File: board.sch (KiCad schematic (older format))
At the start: 32 parts, among them J1 TEMPS, J2 OLED, J3 RELAY, J4 RELAY_EN, J5 USB_B_Micro, Q1 MMBT3904, Q2 MMBT3904, SW1 SW_RESET, U1 ESP32-WROOM-32, U2 AMS1117-3.3, U3 CP2104

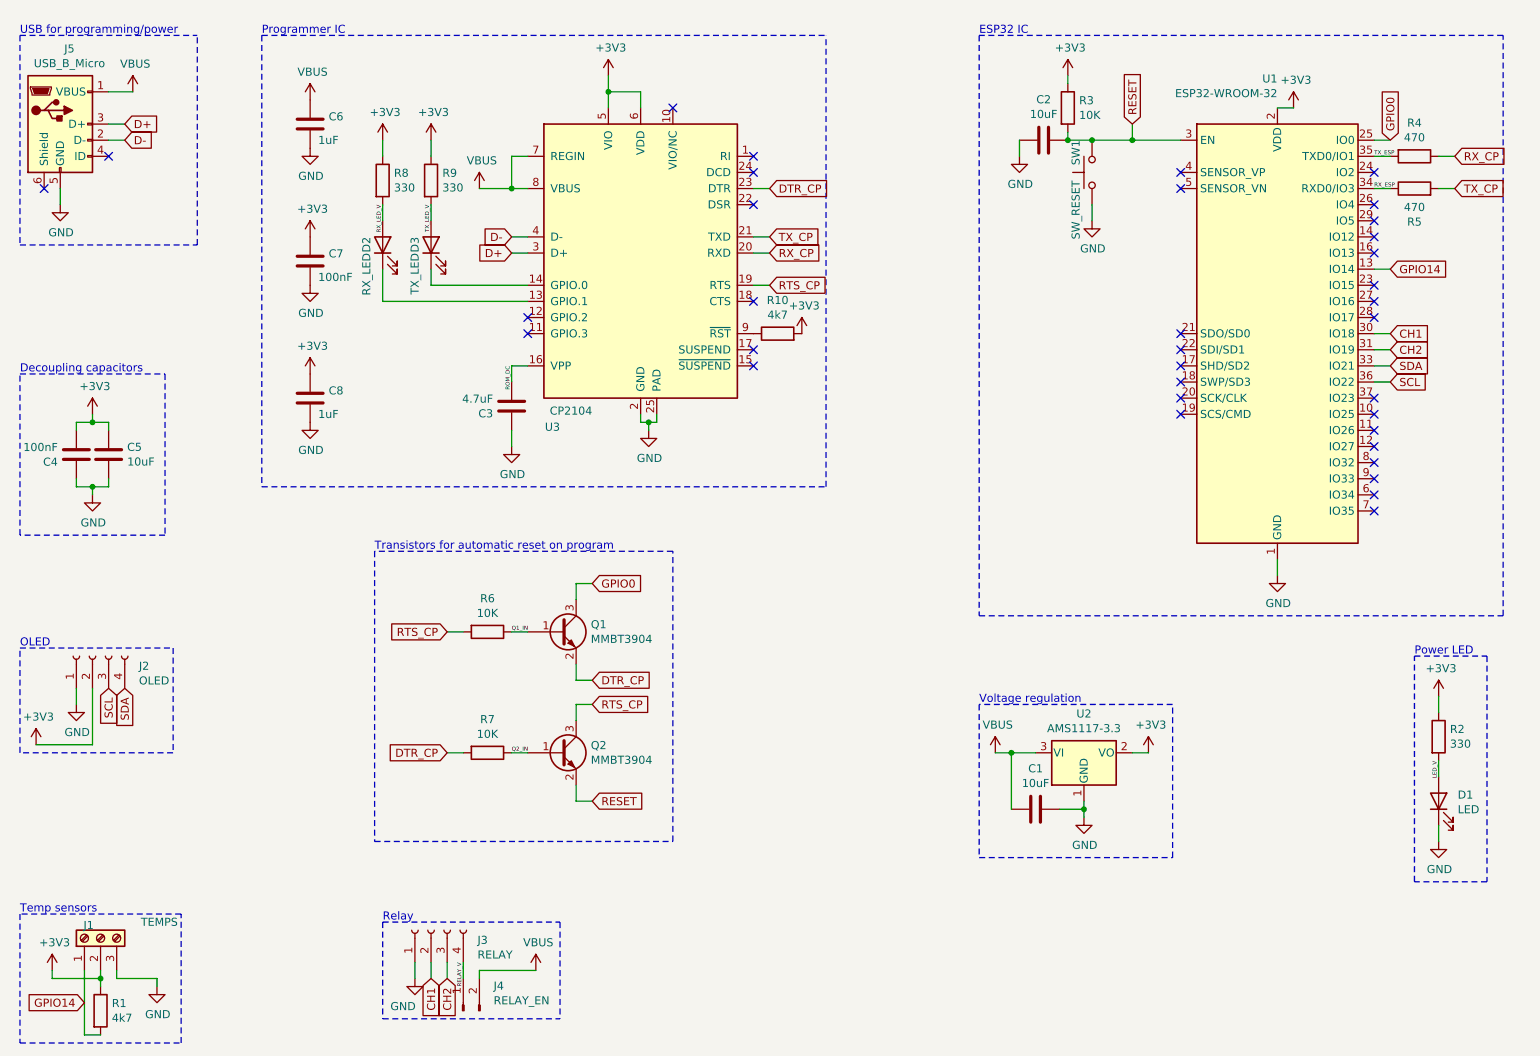
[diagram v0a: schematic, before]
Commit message: with programmer
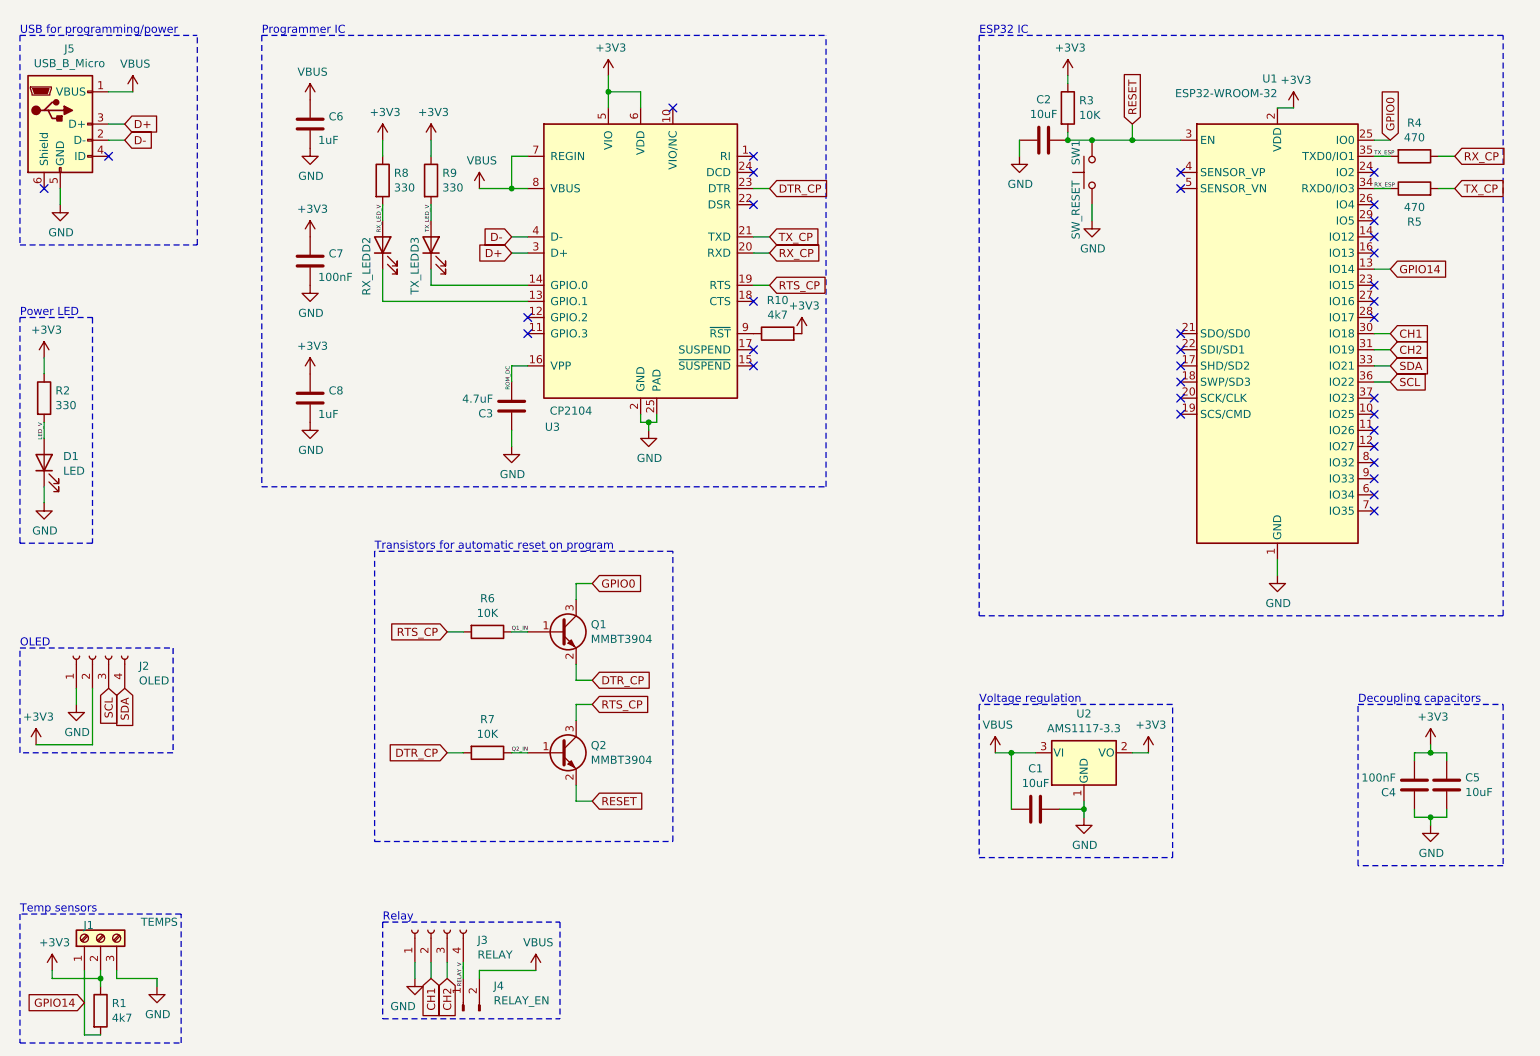
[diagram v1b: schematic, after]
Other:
- moved on the sheet: C4, C5, D1, R2
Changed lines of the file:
@@
 L Device:LED D1
 U 1 1 60E6779F
-P 9750 5700
-F 0 "D1" V 9789 5582 50  0000 R CNN
-F 1 "LED" V 9698 5582 50  0000 R CNN
-F 2 "LED_SMD:LED_0805_2012Metric" H 9750 5700 50  0001 C CNN
-F 3 "~" H 9750 5700 50  0001 C CNN
-	1    9750 5700
+P 1100 3600
+F 0 "D1" V 1139 3482 50  0000 R CNN
+F 1 "LED" V 1048 3482 50  0000 R CNN
+F 2 "LED_SMD:LED_0805_2012Metric" H 1100 3600 50  0001 C CNN
+F 3 "~" H 1100 3600 50  0001 C CNN
+	1    1100 3600
 	0    -1   -1   0
 $EndComp
@@
 L power:+3V3 #PWR01
 U 1 1 60E6985D
-P 9750 5050
-F 0 "#PWR01" H 9750 4900 50  0001 C CNN
-F 1 "+3V3" H 9765 5223 50  0000 C CNN
-F 2 "" H 9750 5050 50  0001 C CNN
-F 3 "" H 9750 5050 50  0001 C CNN
-	1    9750 5050
+P 1100 2950
+F 0 "#PWR01" H 1100 2800 50  0001 C CNN
+F 1 "+3V3" H 1115 3123 50  0000 C CNN
+F 2 "" H 1100 2950 50  0001 C CNN
+F 3 "" H 1100 2950 50  0001 C CNN
+	1    1100 2950
 	1    0    0    -1
 $EndComp
@@
 L Device:R R2
 U 1 1 60E6DB9C
-P 9750 5300
-F 0 "R2" H 9820 5346 50  0000 L CNN
-F 1 "330" H 9820 5255 50  0000 L CNN
-F 2 "Resistor_SMD:R_0805_2012Metric" V 9680 5300 50  0001 C CNN
-F 3 "~" H 9750 5300 50  0001 C CNN
-	1    9750 5300
+P 1100 3200
+F 0 "R2" H 1170 3246 50  0000 L CNN
+F 1 "330" H 1170 3155 50  0000 L CNN
+F 2 "Resistor_SMD:R_0805_2012Metric" V 1030 3200 50  0001 C CNN
+F 3 "~" H 1100 3200 50  0001 C CNN
+	1    1100 3200
 	1    0    0    -1
 $EndComp
@@
 L power:GND #PWR02
 U 1 1 60E6FC7F
-P 9750 5950
-F 0 "#PWR02" H 9750 5700 50  0001 C CNN
-F 1 "GND" H 9755 5777 50  0000 C CNN
-F 2 "" H 9750 5950 50  0001 C CNN
-F 3 "" H 9750 5950 50  0001 C CNN
-	1    9750 5950
-	1    0    0    -1
-$EndComp
-Wire Wire Line
-	9750 5050 9750 5150
-Wire Wire Line
-	9750 5450 9750 5550
-Wire Wire Line
-	9750 5850 9750 5950
-Text Notes 9600 4800 0    50   ~ 0
+P 1100 3850
+F 0 "#PWR02" H 1100 3600 50  0001 C CNN
+F 1 "GND" H 1105 3677 50  0000 C CNN
+F 2 "" H 1100 3850 50  0001 C CNN
+F 3 "" H 1100 3850 50  0001 C CNN
+	1    1100 3850
+	1    0    0    -1
+$EndComp
+Wire Wire Line
+	1100 2950 1100 3050
+Wire Wire Line
+	1100 3350 1100 3450
+Wire Wire Line
+	1100 3750 1100 3850
+Text Notes 950  2700 0    50   ~ 0
 Power LED
 NoConn ~ 9350 1800
@@
 Wire Wire Line
 	7600 2100 7600 2000
-Text Notes 950  3050 0    50   ~ 0
+Text Notes 9250 5100 0    50   ~ 0
 Decoupling capacitors
 $Comp
 L power:GND #PWR0111
 U 1 1 60EBC3E7
-P 1400 3800
-F 0 "#PWR0111" H 1400 3550 50  0001 C CNN
-F 1 "GND" H 1405 3627 50  0000 C CNN
-F 2 "" H 1400 3800 50  0001 C CNN
-F 3 "" H 1400 3800 50  0001 C CNN
-	1    1400 3800
+P 9700 5850
+F 0 "#PWR0111" H 9700 5600 50  0001 C CNN
+F 1 "GND" H 9705 5677 50  0000 C CNN
+F 2 "" H 9700 5850 50  0001 C CNN
+F 3 "" H 9700 5850 50  0001 C CNN
+	1    9700 5850
 	1    0    0    -1
 $EndComp
@@
 L power:+3V3 #PWR0112
 U 1 1 60EBD934
-P 1400 3300
-F 0 "#PWR0112" H 1400 3150 50  0001 C CNN
-F 1 "+3V3" H 1415 3473 50  0000 C CNN
-F 2 "" H 1400 3300 50  0001 C CNN
-F 3 "" H 1400 3300 50  0001 C CNN
-	1    1400 3300
+P 9700 5350
+F 0 "#PWR0112" H 9700 5200 50  0001 C CNN
+F 1 "+3V3" H 9715 5523 50  0000 C CNN
+F 2 "" H 9700 5350 50  0001 C CNN
+F 3 "" H 9700 5350 50  0001 C CNN
+	1    9700 5350
 	1    0    0    -1
 $EndComp
@@
 L Device:C C5
 U 1 1 60EBFBEA
-P 1500 3550
-F 0 "C5" H 1615 3596 50  0000 L CNN
-F 1 "10uF" H 1615 3505 50  0000 L CNN
-F 2 "Capacitor_SMD:C_0805_2012Metric" H 1538 3400 50  0001 C CNN
-F 3 "~" H 1500 3550 50  0001 C CNN
-	1    1500 3550
+P 9800 5600
+F 0 "C5" H 9915 5646 50  0000 L CNN
+F 1 "10uF" H 9915 5555 50  0000 L CNN
+F 2 "Capacitor_SMD:C_0805_2012Metric" H 9838 5450 50  0001 C CNN
+F 3 "~" H 9800 5600 50  0001 C CNN
+	1    9800 5600
 	1    0    0    -1
 $EndComp
@@
 L Device:C C4
 U 1 1 60EC10E0
-P 1300 3550
-F 0 "C4" H 1415 3596 50  0000 L CNN
-F 1 "100nF" H 1415 3505 50  0000 L CNN
-F 2 "Capacitor_SMD:C_0805_2012Metric" H 1338 3400 50  0001 C CNN
-F 3 "~" H 1300 3550 50  0001 C CNN
-	1    1300 3550
+P 9600 5600
+F 0 "C4" H 9715 5646 50  0000 L CNN
+F 1 "100nF" H 9715 5555 50  0000 L CNN
+F 2 "Capacitor_SMD:C_0805_2012Metric" H 9638 5450 50  0001 C CNN
+F 3 "~" H 9600 5600 50  0001 C CNN
+	1    9600 5600
 	-1   0    0    1
 $EndComp
 Wire Wire Line
-	1300 3400 1300 3350
-Wire Wire Line
-	1300 3350 1400 3350
-Wire Wire Line
-	1400 3350 1400 3300
-Wire Wire Line
-	1500 3400 1500 3350
-Wire Wire Line
-	1500 3350 1400 3350
-Connection ~ 1400 3350
-Wire Wire Line
-	1300 3700 1300 3750
-Wire Wire Line
-	1300 3750 1400 3750
-Wire Wire Line
-	1400 3750 1400 3800
-Wire Wire Line
-	1500 3700 1500 3750
-Wire Wire Line
-	1500 3750 1400 3750
-Connection ~ 1400 3750
+	9600 5450 9600 5400
+Wire Wire Line
+	9600 5400 9700 5400
+Wire Wire Line
+	9700 5400 9700 5350
+Wire Wire Line
+	9800 5450 9800 5400
+Wire Wire Line
+	9800 5400 9700 5400
+Connection ~ 9700 5400
+Wire Wire Line
+	9600 5750 9600 5800
+Wire Wire Line
+	9600 5800 9700 5800
+Wire Wire Line
+	9700 5800 9700 5850
+Wire Wire Line
+	9800 5750 9800 5800
+Wire Wire Line
+	9800 5800 9700 5800
+Connection ~ 9700 5800
 $Comp
 L Device:R R4
@@
 Transistors for automatic reset on program
 Wire Notes Line
-	1850 3050 1850 4050
-Wire Notes Line
-	1850 4050 950  4050
-Wire Notes Line
-	950  4050 950  3050
-Wire Notes Line
-	950  3050 1850 3050
+	10150 5100 10150 6100
+Wire Notes Line
+	10150 6100 9250 6100
+Wire Notes Line
+	9250 6100 9250 5100
+Wire Notes Line
+	9250 5100 10150 5100
 Wire Notes Line
 	5950 3750 5950 950
@@
 Programmer IC
 Wire Notes Line
-	10050 4800 10050 6200
-Wire Notes Line
-	10050 6200 9600 6200
-Wire Notes Line
-	9600 6200 9600 4800
-Wire Notes Line
-	9600 4800 10050 4800
+	1400 2700 1400 4100
+Wire Notes Line
+	1400 4100 950  4100
+Wire Notes Line
+	950  4100 950  2700
+Wire Notes Line
+	950  2700 1400 2700
 Wire Notes Line
 	950  950  950  2250
@@
 Wire Notes Line
 	8100 5100 6900 5100
-Text Label 9750 5450 3    25   ~ 0
+Text Label 1100 3350 3    25   ~ 0
 LED_V
 Text Label 4000 5400 0    25   ~ 0

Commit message: initial finished board pre-fab
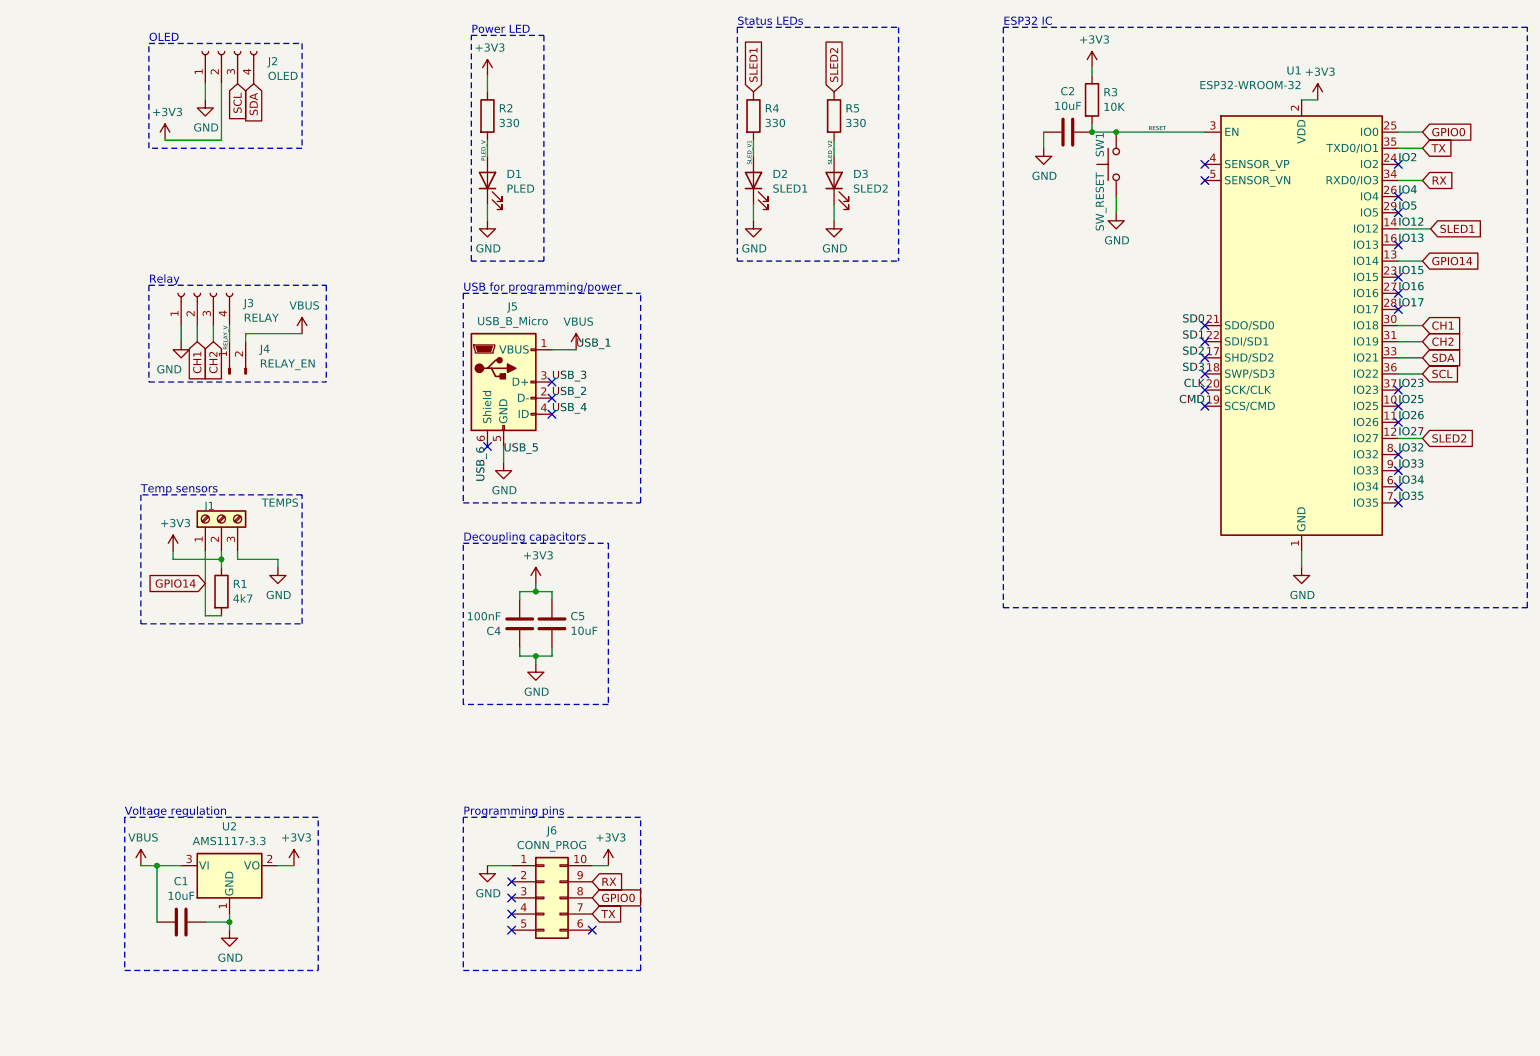
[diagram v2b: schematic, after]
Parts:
- removed C3: 4.7uF, Capacitor_SMD:C_0805_2012Metric, symbol Device:C
- removed C6, C8: 1uF, Capacitor_SMD:C_0805_2012Metric, symbol Device:C
- removed C7: 100nF, Capacitor_SMD:C_0805_2012Metric, symbol Device:C
- removed Q1, Q2: MMBT3904, Package_TO_SOT_SMD:SOT-23, symbol Transistor_BJT:MMBT3904
- removed R10: 4k7, Resistor_SMD:R_0805_2012Metric, symbol Device:R
- removed R6, R7: 10K, Resistor_SMD:R_0805_2012Metric, symbol Device:R
- removed R8, R9: 330, Resistor_SMD:R_0805_2012Metric, symbol Device:R
- removed U3: CP2104, Package_DFN_QFN:QFN-24-1EP_4x4mm_P0.5mm_EP2.6x2.6mm, symbol Interface_USB:CP2104
- added J6: CONN_PROG, Connector_PinHeader_1.27mm:PinHeader_2x05_P1.27mm_Vertical_SMD, symbol Connector_Generic:Conn_02x05_Counter_Clockwise
- D1: value LED -> PLED
- D2: value RX_LED -> SLED1
- D3: value TX_LED -> SLED2
- R4, R5: value 470 -> 330
- U1: Part No (none) -> C82899
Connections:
- net RX_CP is gone; now on net SLED1: R4.1
- net TX_LED_V is gone; now on net SLED_V2: D3.2 (A)
- net +3V3: now also J6.10 (Pin_10)
- net GND: now also D2.1 (K), D3.1 (K), J6.1 (Pin_1)
- net GPIO0: now also J6.8 (Pin_8)
- net IO25: now reaches U1.10 (IO25)
- net IO26: now reaches U1.11 (IO26)
- net SLED2: now reaches U1.12 (IO27)
- net SLED2: now also R5.1
- net SLED1: now reaches U1.14 (IO12)
- net IO13: now reaches U1.16 (IO13)
- net SD2: now reaches U1.17 (SHD/SD2)
- net SD3: now reaches U1.18 (SWP/SD3)
- net CMD: now reaches U1.19 (SCS/CMD)
- net CLK: now reaches U1.20 (SCK/CLK)
- net SD0: now reaches U1.21 (SDO/SD0)
- net SD1: now reaches U1.22 (SDI/SD1)
- net IO15: now reaches U1.23 (IO15)
- net IO2: now reaches U1.24 (IO2)
- net IO4: now reaches U1.26 (IO4)
- net IO16: now reaches U1.27 (IO16)
- net IO17: now reaches U1.28 (IO17)
- net IO5: now reaches U1.29 (IO5)
- net IO23: now reaches U1.37 (IO23)
- net IO34: now reaches U1.6 (IO34)
- net IO35: now reaches U1.7 (IO35)
- net IO32: now reaches U1.8 (IO32)
- net IO33: now reaches U1.9 (IO33)
- net USB_4: now reaches J5.4 (ID)
- net USB_6: now reaches J5.6 (Shield)
- net D+ renamed USB_3
- net D- renamed USB_2
- net LED_V renamed PLED_V
- net RX_ESP renamed RX
- net RX: now also J6.9 (Pin_9); no longer R5.1
- net RX_LED_V renamed SLED_V1
- net SLED_V1: now also R4.2
- net TX_CP renamed SLED_V2
- net TX_ESP renamed TX
- net TX: now also J6.7 (Pin_7); no longer R4.2
- no-connect marks 35 -> 31
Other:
- note added: "Programming pins"
- note added: "Status LEDs"
- note removed: "Programmer IC"
- note removed: "Transistors for automatic reset on program"
- moved on the sheet: C1, C2, C4, C5, D1, J1, J2, J3, J4, J5, R1, R2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
